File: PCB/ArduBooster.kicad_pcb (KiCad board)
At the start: 2 copper layers, 74.9 x 50 mm, 30 parts, among them IC1 ATMEGA328-P, P1 ISP, P2 DEBUG TX/RX, P3 CONTROL, P4 MAIN_CONN, U1 ICL7660, U2 LM358, U3 4052, X1 CRYSTAL

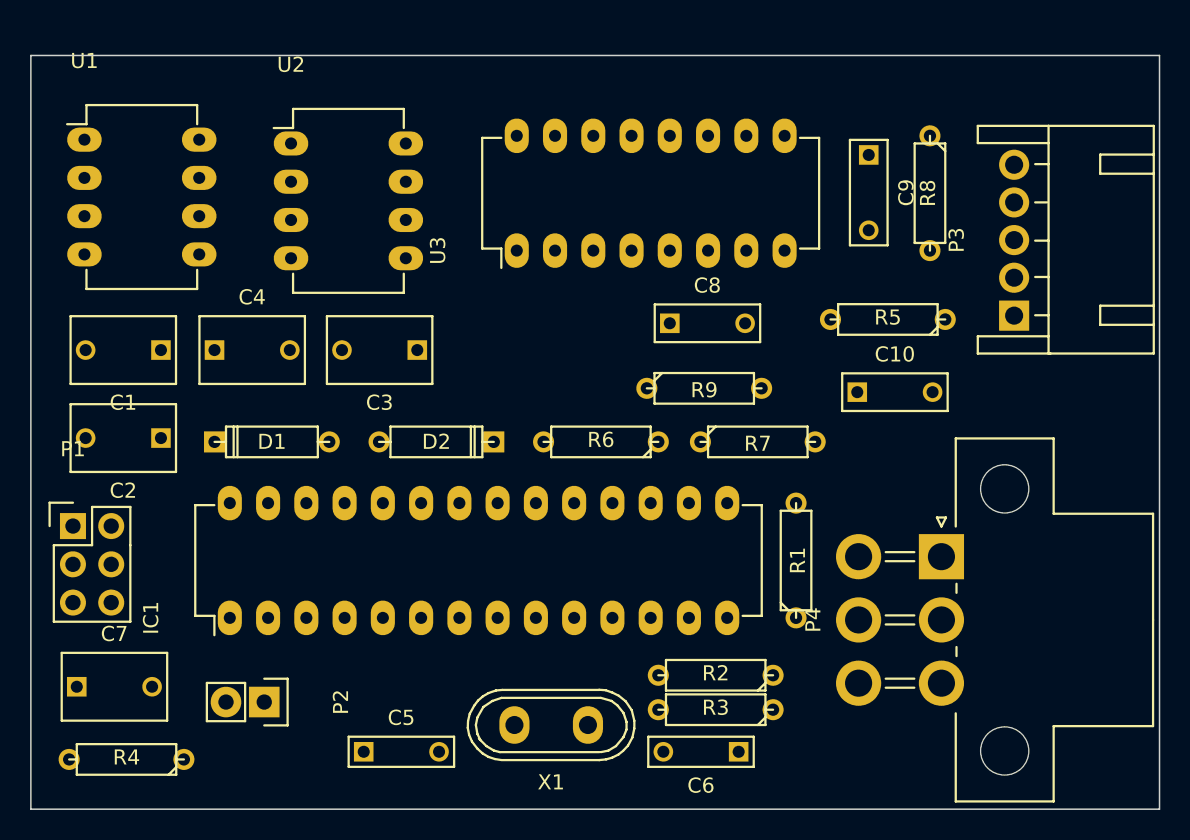
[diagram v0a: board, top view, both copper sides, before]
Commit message: Routing...
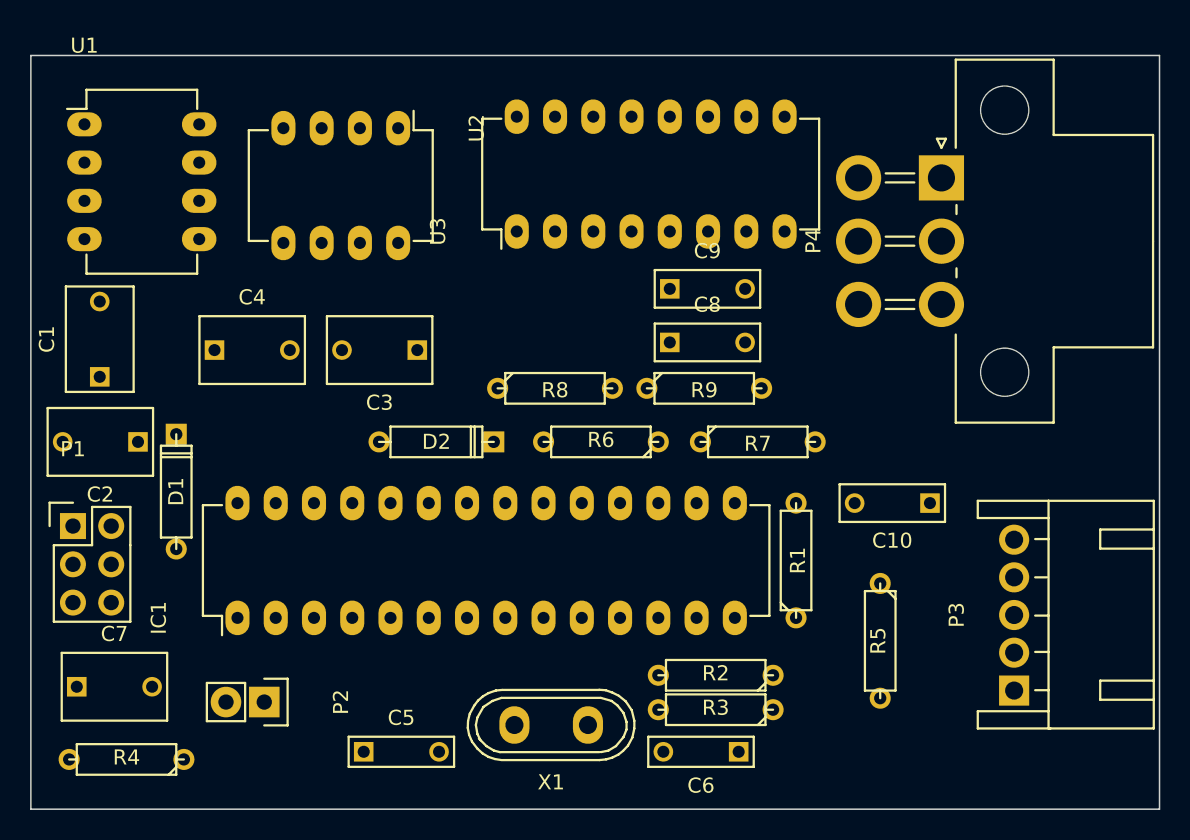
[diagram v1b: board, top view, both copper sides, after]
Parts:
- moved R8 28.1 mm to (140.5, 58.9), turned to 0 degrees
- moved P4 25.1 mm to (166.1, 45.0)
- moved P3 24.9 mm to (170.9, 79.0)
- moved R5 21.3 mm to (162.1, 75.7), turned to 270 degrees
- moved C9 15.9 mm to (148.1, 52.3), turned to 0 degrees
- moved C10 8.81 mm to (165.4, 66.5), turned to 180 degrees
- moved U2 7.18 mm to (130.0, 41.7), turned to 270 degrees
- moved D1 7.16 mm to (115.3, 65.8), turned to 90 degrees
- moved C1 4.44 mm to (110.2, 58.2), turned to 90 degrees
- moved C2 1.55 mm to (112.8, 62.5)
- moved C8 1.27 mm to (148.1, 55.9)
- moved U3 1.27 mm to (137.9, 48.5)
- moved U1 1.02 mm to (109.2, 41.4)
- moved IC1 0.51 mm to (119.4, 74.2)
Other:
- net class Default: clearance 0.5 -> 0.3; trace_width 0.6 -> 0.3
- rule trace_clearance: 0.5 -> 0.3
